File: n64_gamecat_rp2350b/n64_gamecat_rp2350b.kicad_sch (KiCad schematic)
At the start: 6 parts, among them J1 Conn_01x03_Pin, J2 Conn_01x03_Pin, J3 Conn_01x05, U4 RP235x-B

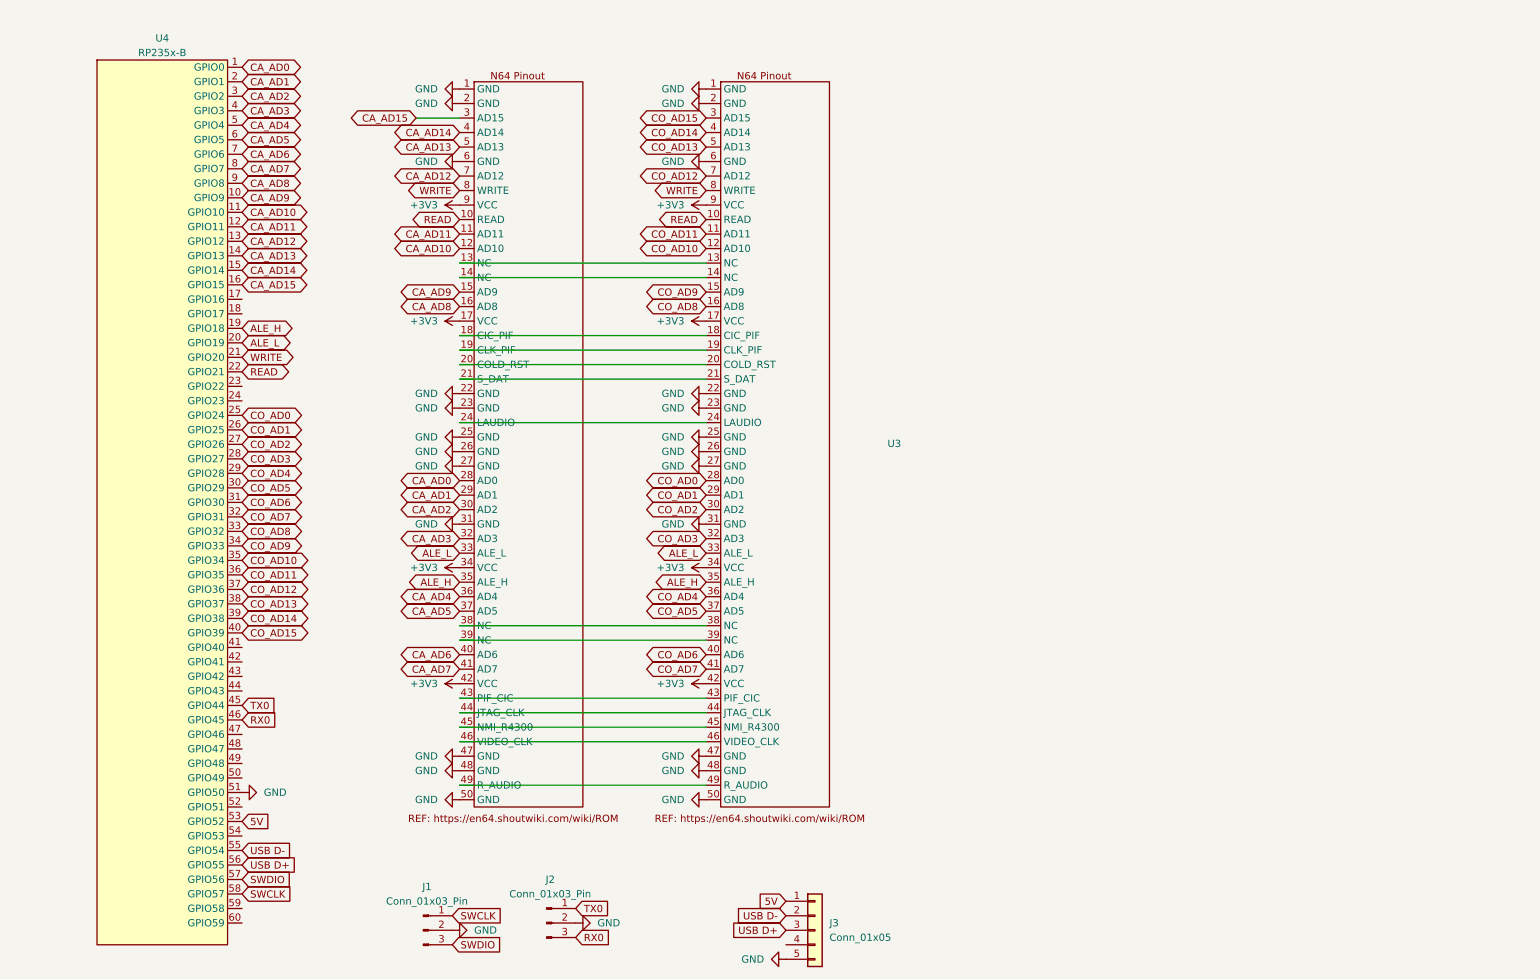
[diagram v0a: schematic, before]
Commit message: Misc changes; add OoT decomp
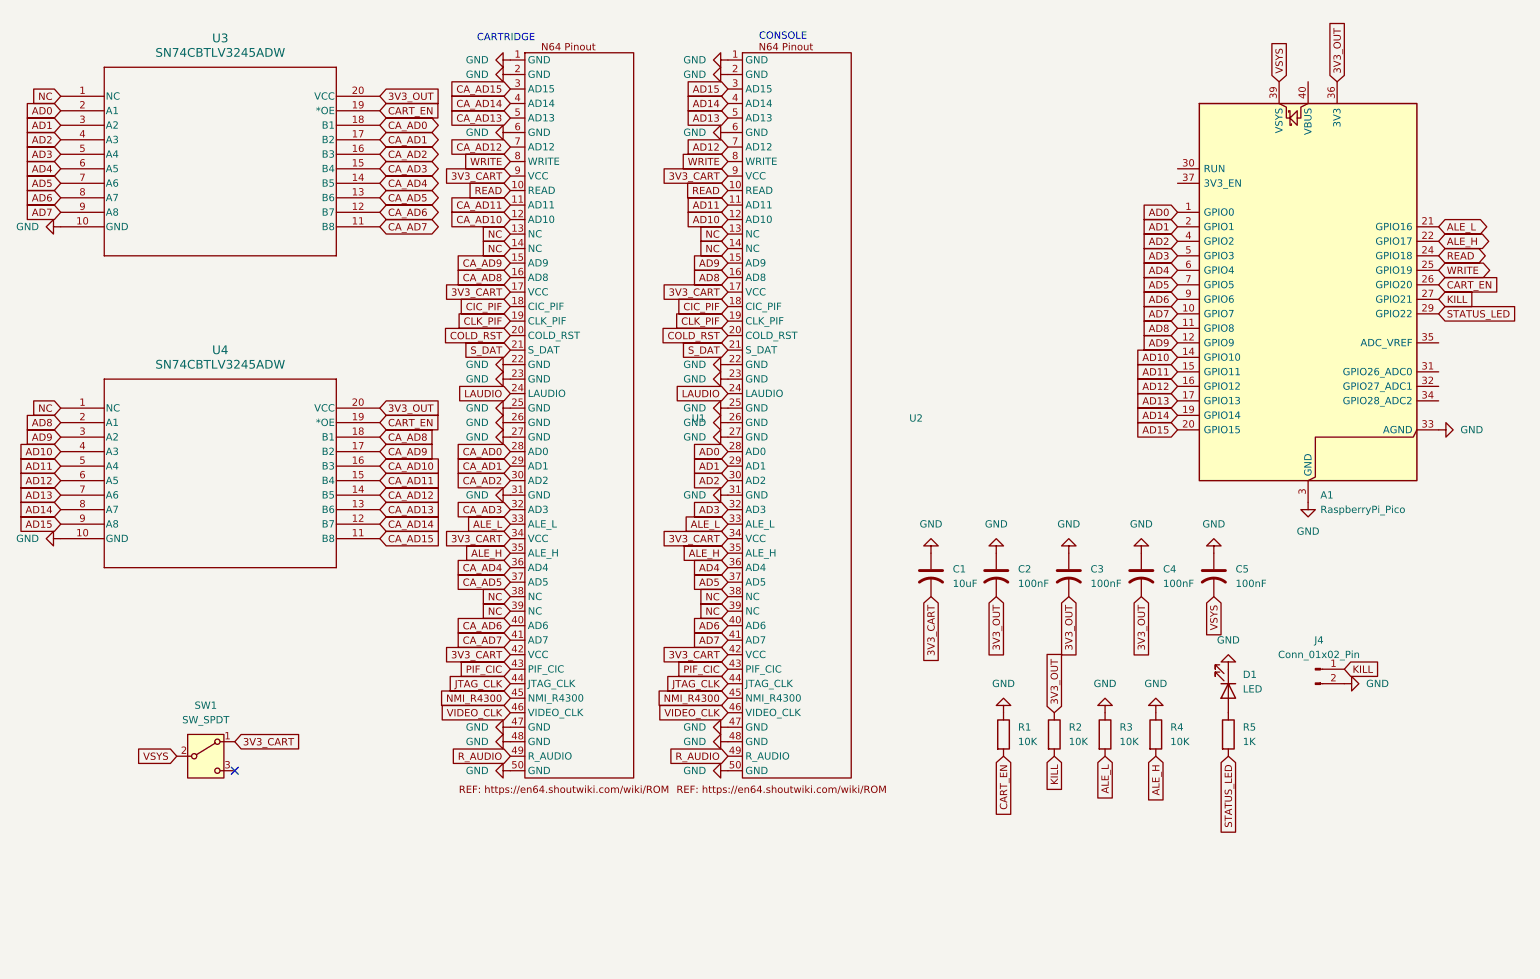
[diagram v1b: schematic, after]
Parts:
- removed J1, J2: Conn_01x03_Pin, Connector_PinHeader_2.54mm:PinHeader_1x03_P2.54mm_Vertical, symbol Connector:Conn_01x03_Pin
- removed J3: Conn_01x05, Connector_PinSocket_2.54mm:PinSocket_1x05_P2.54mm_Vertical, symbol Connector_Generic:Conn_01x05
- removed U2: ~, n64_library:N64_cartridge_connecter_2.5mm, symbol n64:cartridge_connector
- removed U3: ~, n64_library:N64_cartridge_pins_2.5mm, symbol n64:console_connector
- removed U4: RP235x-B, RP2xxx_Stamp:RP2xxx_Stamp_XL_THT, symbol MCU_RaspberryPi2:RP2350B_Stamp_XL
- added A1: RaspberryPi_Pico, Module:RaspberryPi_Pico_Common_Unspecified, symbol MCU_Module:RaspberryPi_Pico
- added C1: 10uF, Capacitor_SMD:C_0805_2012Metric, symbol Device:C_US
- added C2, C3, C4, C5: 100nF, Capacitor_SMD:C_0402_1005Metric, symbol Device:C_US
- added D1: LED, LED_SMD:LED_0402_1005Metric, symbol Device:LED
- added J4: Conn_01x02_Pin, Connector_PinHeader_2.54mm:PinHeader_1x02_P2.54mm_Vertical, symbol Connector:Conn_01x02_Pin
- added R1, R2, R3, R4: 10K, Resistor_SMD:R_0402_1005Metric, symbol Device:R
- added R5: 1K, Resistor_SMD:R_0402_1005Metric, symbol Device:R
- added SW1: SW_SPDT, Connector_PinSocket_2.54mm:PinSocket_1x03_P2.54mm_Vertical, symbol Switch:SW_SPDT
- added U1: (no value), n64_library:N64_cartridge_connecter_2.5mm, symbol n64:cartridge_connector
- added U2: (no value), n64_library:N64_cartridge_pins_2.5mm, symbol n64:console_connector
- added U3, U4: SN74CBTLV3245ADW, footprints:DW20, symbol 2026-04-17_18-55-28:SN74CBTLV3245ADW
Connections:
- net ALE_H: now also A1.22 (GPIO17), R4.2, U1.35 (ALE_H), U2.35 (ALE_H)
- net ALE_L: now also A1.21 (GPIO16), R3.2, U1.33 (ALE_L), U2.33 (ALE_L)
- net CA_AD0: now also U1.28 (AD0), U3.18 (B1)
- net CA_AD1: now also U1.29 (AD1), U3.17 (B2)
- net CA_AD10: now also U1.12 (AD10), U4.16 (B3)
- net CA_AD11: now also U1.11 (AD11), U4.15 (B4)
- net CA_AD12: now also U1.7 (AD12), U4.14 (B5)
- net CA_AD13: now also U1.5 (AD13), U4.13 (B6)
- net CA_AD14: now also U1.4 (AD14), U4.12 (B7)
- net CA_AD15: now also U1.3 (AD15), U4.11 (B8)
- net CA_AD2: now also U1.30 (AD2), U3.16 (B3)
- net CA_AD3: now also U1.32 (AD3), U3.15 (B4)
- net CA_AD4: now also U1.36 (AD4), U3.14 (B5)
- net CA_AD5: now also U1.37 (AD5), U3.13 (B6)
- net CA_AD6: now also U1.40 (AD6), U3.12 (B7)
- net CA_AD7: now also U1.41 (AD7), U3.11 (B8)
- net CA_AD8: now also U1.16 (AD8), U4.18 (B1)
- net CA_AD9: now also U1.15 (AD9), U4.17 (B2)
- net GND: now also A1.13 (GND), A1.18 (GND), A1.23 (GND), A1.28 (GND), A1.3 (GND), A1.33 (AGND), A1.38 (GND), A1.8 (GND), C1.1, C2.1, C3.1, C4.1, C5.1, D1.1 (K), J4.2 (Pin_2), R1.1, R3.1, R4.1, U1.1 (GND), U1.2 (GND), U1.22 (GND), U1.23 (GND), U1.25 (GND), U1.26 (GND), U1.27 (GND), U1.31 (GND), U1.47 (GND), U1.48 (GND), U1.50 (GND), U1.6 (GND), U2.1 (GND), U2.2 (GND), U2.22 (GND), U2.23 (GND), U2.25 (GND), U2.26 (GND), U2.27 (GND), U2.31 (GND), U2.47 (GND), U2.48 (GND), U2.50 (GND), U2.6 (GND), U3.10 (GND), U4.10 (GND)
- net READ: now also A1.24 (GPIO18), U1.10 (READ), U2.10 (READ)
- net WRITE: now also A1.25 (GPIO19), U1.8 (WRITE), U2.8 (WRITE)
- new net: D1.2 (A), R5.1
- new net 3V3_CART: C1.2, SW1.1 (A), U1.17 (VCC), U1.34 (VCC), U1.42 (VCC), U1.9 (VCC), U2.17 (VCC), U2.34 (VCC), U2.42 (VCC), U2.9 (VCC)
- new net 3V3_OUT: A1.36 (3V3), C2.2, C3.2, C4.2, R2.1, U3.20 (VCC), U4.20 (VCC)
- new net AD0: A1.1 (GPIO0), U2.28 (AD0), U3.2 (A1)
- new net AD1: A1.2 (GPIO1), U2.29 (AD1), U3.3 (A2)
- new net AD10: A1.14 (GPIO10), U2.12 (AD10), U4.4 (A3)
- new net AD11: A1.15 (GPIO11), U2.11 (AD11), U4.5 (A4)
- new net AD12: A1.16 (GPIO12), U2.7 (AD12), U4.6 (A5)
- new net AD13: A1.17 (GPIO13), U2.5 (AD13), U4.7 (A6)
- new net AD14: A1.19 (GPIO14), U2.4 (AD14), U4.8 (A7)
- new net AD15: A1.20 (GPIO15), U2.3 (AD15), U4.9 (A8)
- new net AD2: A1.4 (GPIO2), U2.30 (AD2), U3.4 (A3)
- new net AD3: A1.5 (GPIO3), U2.32 (AD3), U3.5 (A4)
- new net AD4: A1.6 (GPIO4), U2.36 (AD4), U3.6 (A5)
- new net AD5: A1.7 (GPIO5), U2.37 (AD5), U3.7 (A6)
- new net AD6: A1.9 (GPIO6), U2.40 (AD6), U3.8 (A7)
- new net AD7: A1.10 (GPIO7), U2.41 (AD7), U3.9 (A8)
- new net AD8: A1.11 (GPIO8), U2.16 (AD8), U4.2 (A1)
- new net AD9: A1.12 (GPIO9), U2.15 (AD9), U4.3 (A2)
- new net CART_EN: A1.26 (GPIO20), R1.2, U3.19 (*OE), U4.19 (*OE)
- new net CIC_PIF: U1.18 (CIC_PIF), U2.18 (CIC_PIF)
- new net CLK_PIF: U1.19 (CLK_PIF), U2.19 (CLK_PIF)
- new net COLD_RST: U1.20 (COLD_RST), U2.20 (COLD_RST)
- new net JTAG_CLK: U1.44 (JTAG_CLK), U2.44 (JTAG_CLK)
- new net KILL: A1.27 (GPIO21), J4.1 (Pin_1), R2.2
- new net LAUDIO: U1.24 (LAUDIO), U2.24 (LAUDIO)
- new net NC: U1.13 (NC), U1.14 (NC), U1.38 (NC), U1.39 (NC), U2.13 (NC), U2.14 (NC), U2.38 (NC), U2.39 (NC), U3.1 (NC), U4.1 (NC)
- new net NMI_R4300: U1.45 (NMI_R4300), U2.45 (NMI_R4300)
- new net PIF_CIC: U1.43 (PIF_CIC), U2.43 (PIF_CIC)
- new net R_AUDIO: U1.49 (R_AUDIO), U2.49 (R_AUDIO)
- new net STATUS_LED: A1.29 (GPIO22), R5.2
- new net S_DAT: U1.21 (S_DAT), U2.21 (S_DAT)
- new net VIDEO_CLK: U1.46 (VIDEO_CLK), U2.46 (VIDEO_CLK)
- new net VSYS: A1.39 (VSYS), C5.2, SW1.2 (B)
- no-connect marks 0 -> 1
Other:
- note added: "CARTRIDGE"
- note added: "CONSOLE"
